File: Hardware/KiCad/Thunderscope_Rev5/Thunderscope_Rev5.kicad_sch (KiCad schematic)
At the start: 34 parts, among them J1 BNC, J11 7792, J2 BNC, J3 1.27mm 6 Pin TH, J4 TSW-101-16-G-Q-RA, U1 SN74LVC1G17

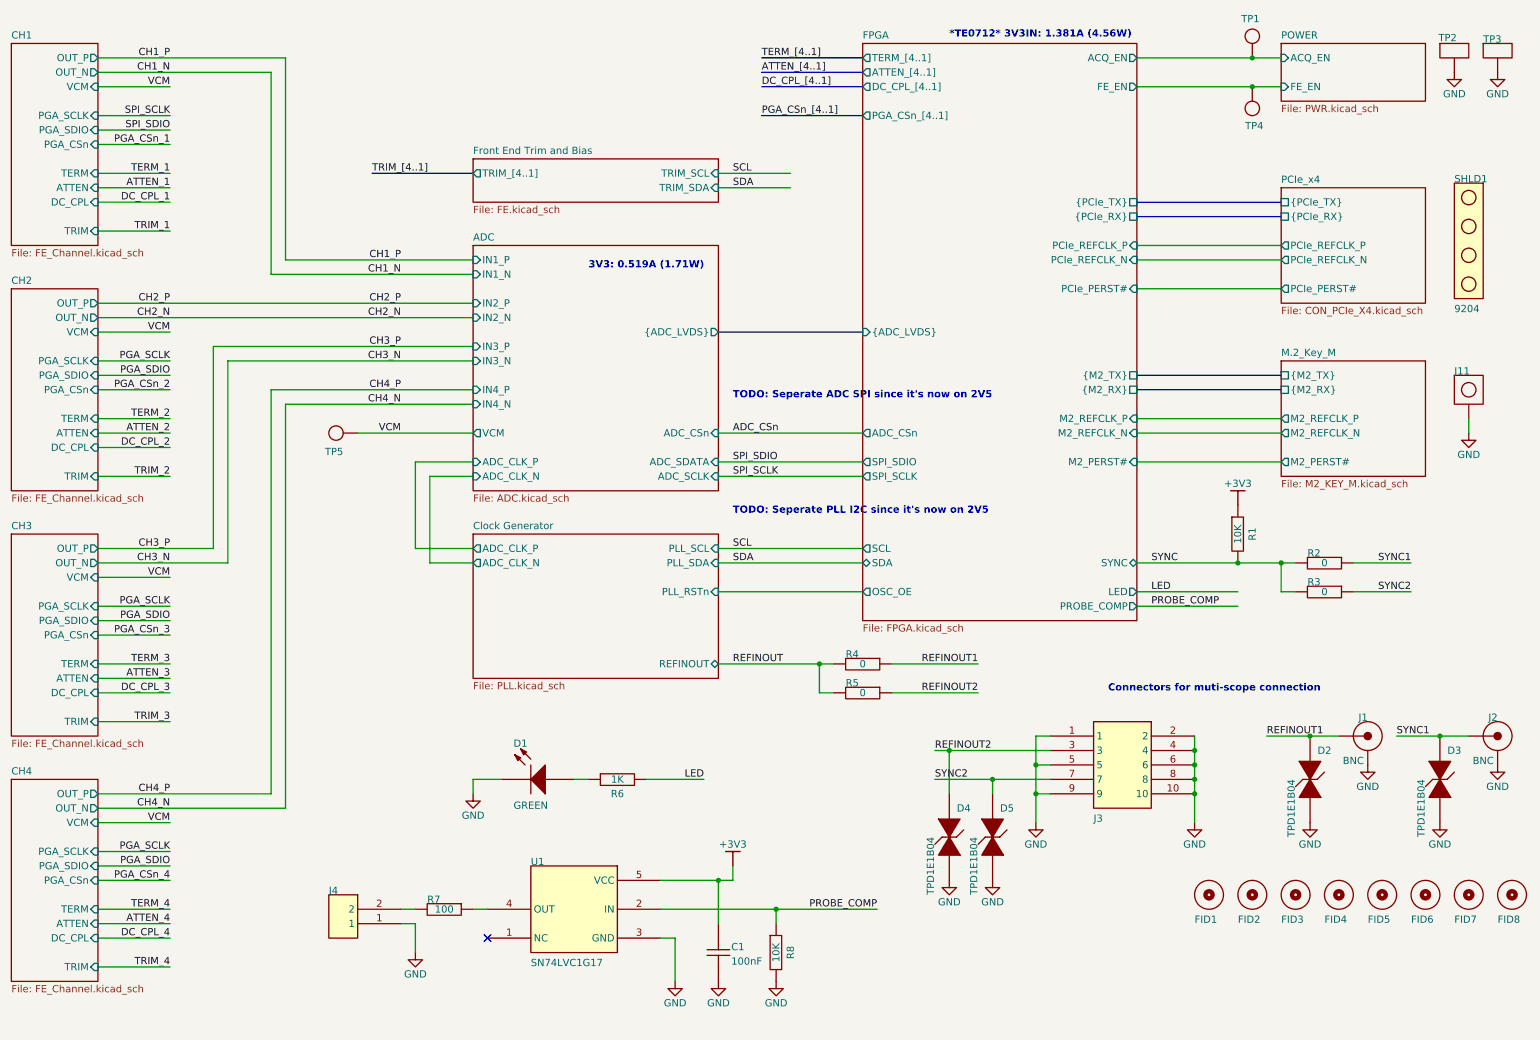
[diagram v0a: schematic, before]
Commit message: Altium Param Import with Script
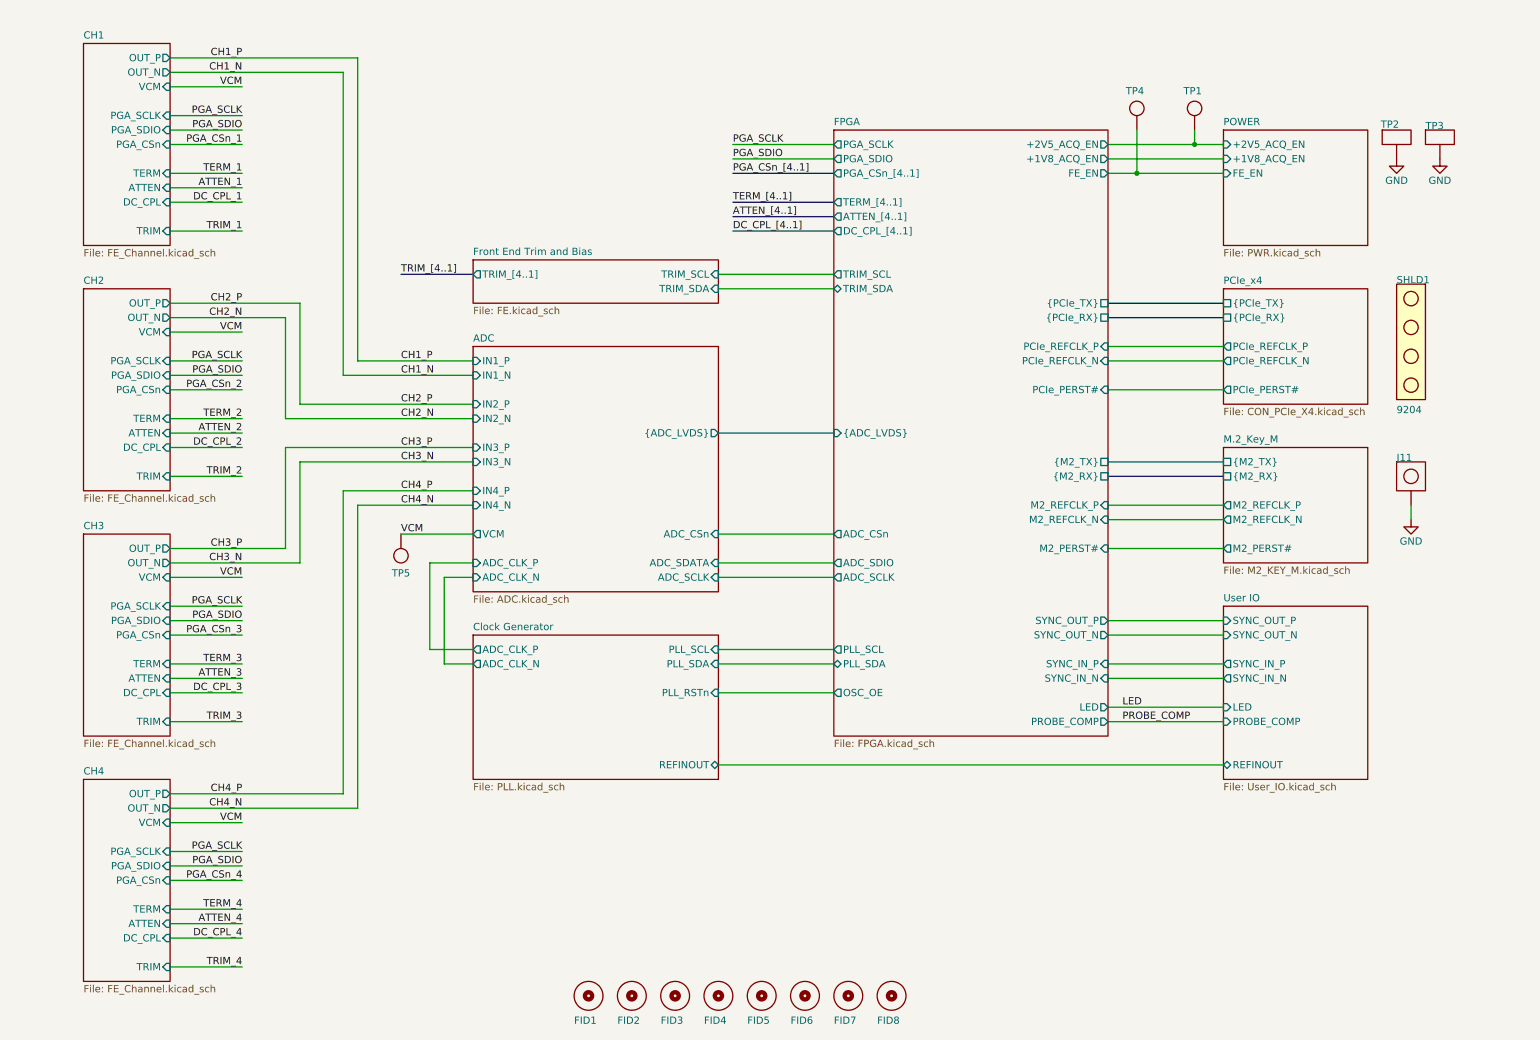
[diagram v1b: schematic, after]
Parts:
- removed C1: ${ALTIUM_VALUE}, GEN_C_0402, symbol Thunderscope_Rev5:CAP 100nF 16V X7R 0402
- removed D1: GREEN, LED_0603_LTST-S270K, symbol Thunderscope_Rev5:LED GREEN 0603 LTST-S270K
- removed D2, D3, D4, D5: TPD1E1B04, TI_X1SON_DPY0002A, symbol Thunderscope_Rev5:TVS TPD1E1B04
- removed J1, J2: BNC, MOL_0731000105, symbol Thunderscope_Rev5:BNC JACK R/A
- removed J3: 1.27mm 6 Pin TH, GEN_1.27mm_2x5_Pin_TH_RA, symbol Thunderscope_Rev5:CONN 1.27mm 2x5 Pin TH RA
- removed J4: TSW-101-16-G-Q-RA, GEN_5.08mm_1x2_Pin_TH_RA, symbol Thunderscope_Rev5:CONN 5.08mm 2 Pin TH RA
- removed R1, R8: ${ALTIUM_VALUE}, GEN_R_0402, symbol Thunderscope_Rev5:RES 10K OHM 1% 1/10W 0402
- removed R2, R3, R4, R5: ${ALTIUM_VALUE}, GEN_R_0402, symbol Thunderscope_Rev5:RES 0 OHM 1/16W 0402
- removed R6: ${ALTIUM_VALUE}, GEN_R_0402, symbol Thunderscope_Rev5:RES 1K OHM 1% 1/10W 0402
- removed R7: ${ALTIUM_VALUE}, GEN_R_0402, symbol Thunderscope_Rev5:RES 100 OHM 1% 1/10W 0402
- removed U1: SN74LVC1G17, GEN_SC-70-5, symbol Thunderscope_Rev5:IC BUFFER SN74LVC1G17
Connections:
- net FPGA/ACQ_EN renamed FPGA/+2V5_ACQ_EN
- no-connect marks 1 -> 0
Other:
- added sheet User IO (User_IO.kicad_sch)
- sheet FPGA ports: added +1V8_ACQ_EN, +2V5_ACQ_EN, ADC_SCLK, ADC_SDIO, PGA_SCLK, PGA_SDIO, PLL_SCL, PLL_SDA, SYNC_IN_N, SYNC_IN_P, SYNC_OUT_N, SYNC_OUT_P, TRIM_SCL, TRIM_SDA; removed ACQ_EN, SCL, SDA, SPI_SCLK, SPI_SDIO, SYNC
- sheet POWER ports: added +1V8_ACQ_EN, +2V5_ACQ_EN; removed ACQ_EN
- note removed: "*TE0712* 3V3IN: 1.381A (4.56W)"
- note removed: "3V3: 0.519A (1.71W)"
- note removed: "Connectors for muti-scope connection"
- note removed: "TODO: Seperate ADC SPI since it's now on 2V5"
- note removed: "TODO: Seperate PLL I2C since it's now on 2V5"
- moved on the sheet: FID1, FID2, FID3, FID4, FID5, FID6, FID7, FID8, J11, SHLD1, TP1, TP2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
